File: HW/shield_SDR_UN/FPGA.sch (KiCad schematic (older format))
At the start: 71 parts, among them J1 Conn_02x09_Odd_Even, J2 Conn_02x08_Odd_Even, U4 XC6SLX9-2TQG144C, X2 ASE-xxxMHz

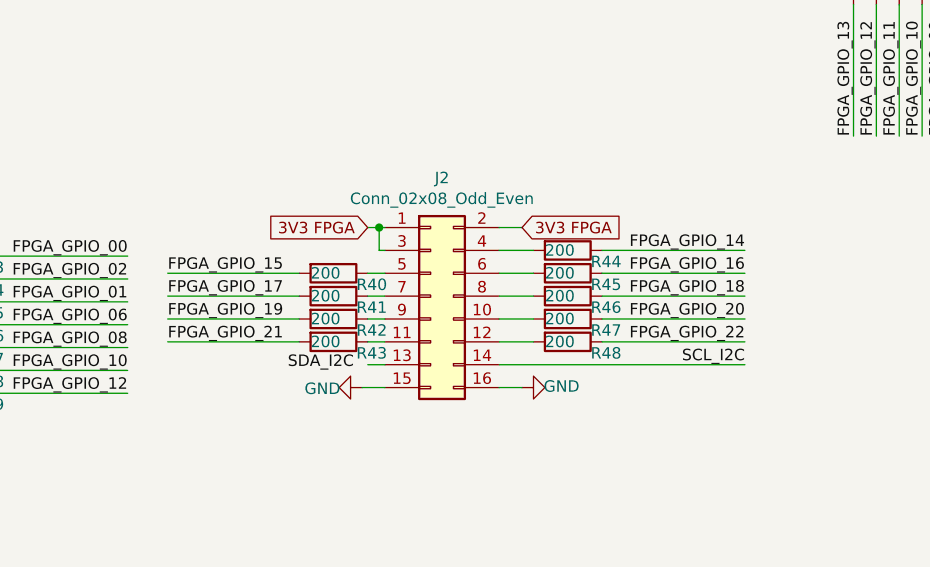
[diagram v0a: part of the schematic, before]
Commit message: organizacion PCB
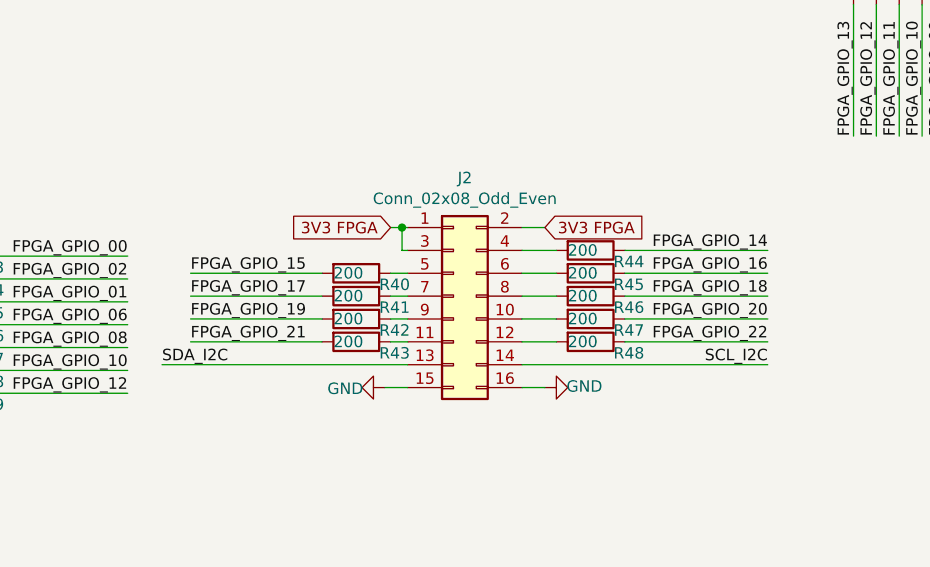
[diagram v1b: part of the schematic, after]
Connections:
- net I2C_SDA: now also J2.13 (Pin_13)
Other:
- moved on the sheet: J2, R40, R41, R42, R43, R44, R45, R46, R47, R48

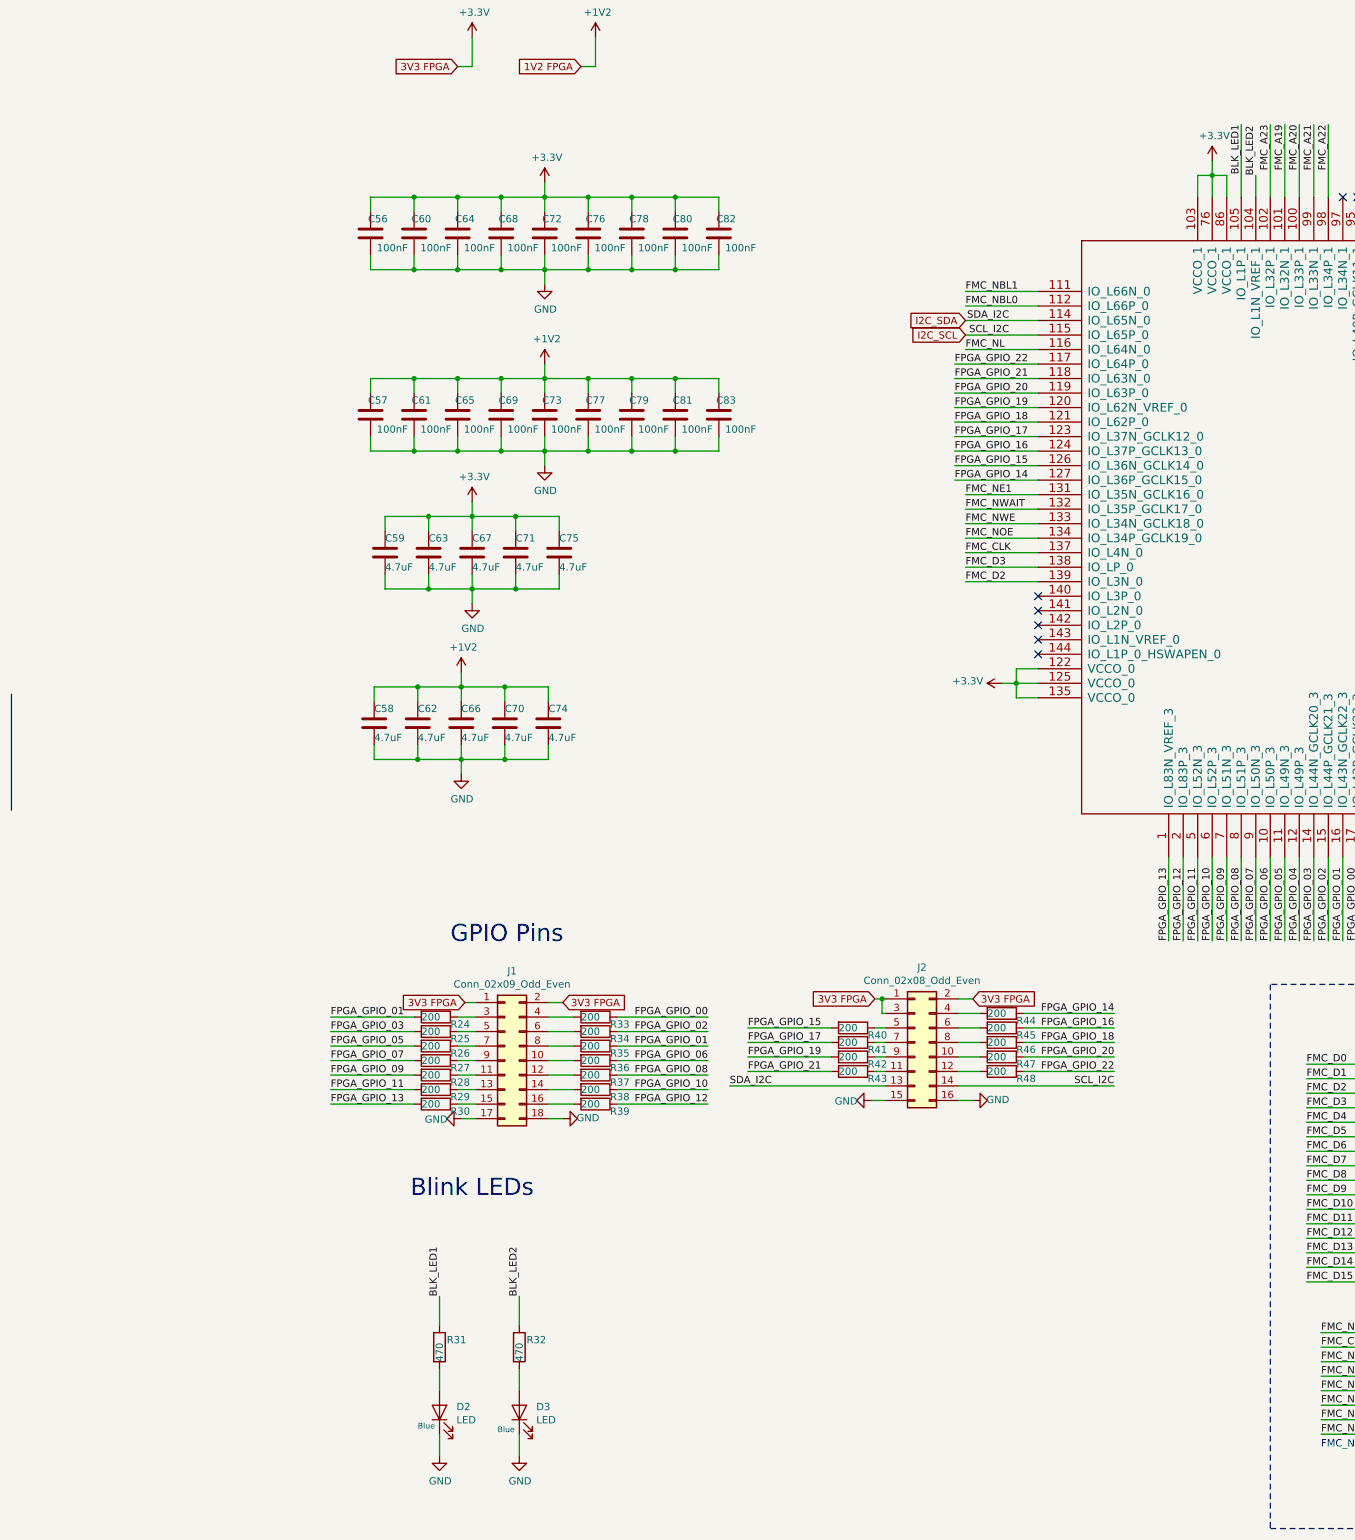
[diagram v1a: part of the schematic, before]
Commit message: organizacion PCB_V2
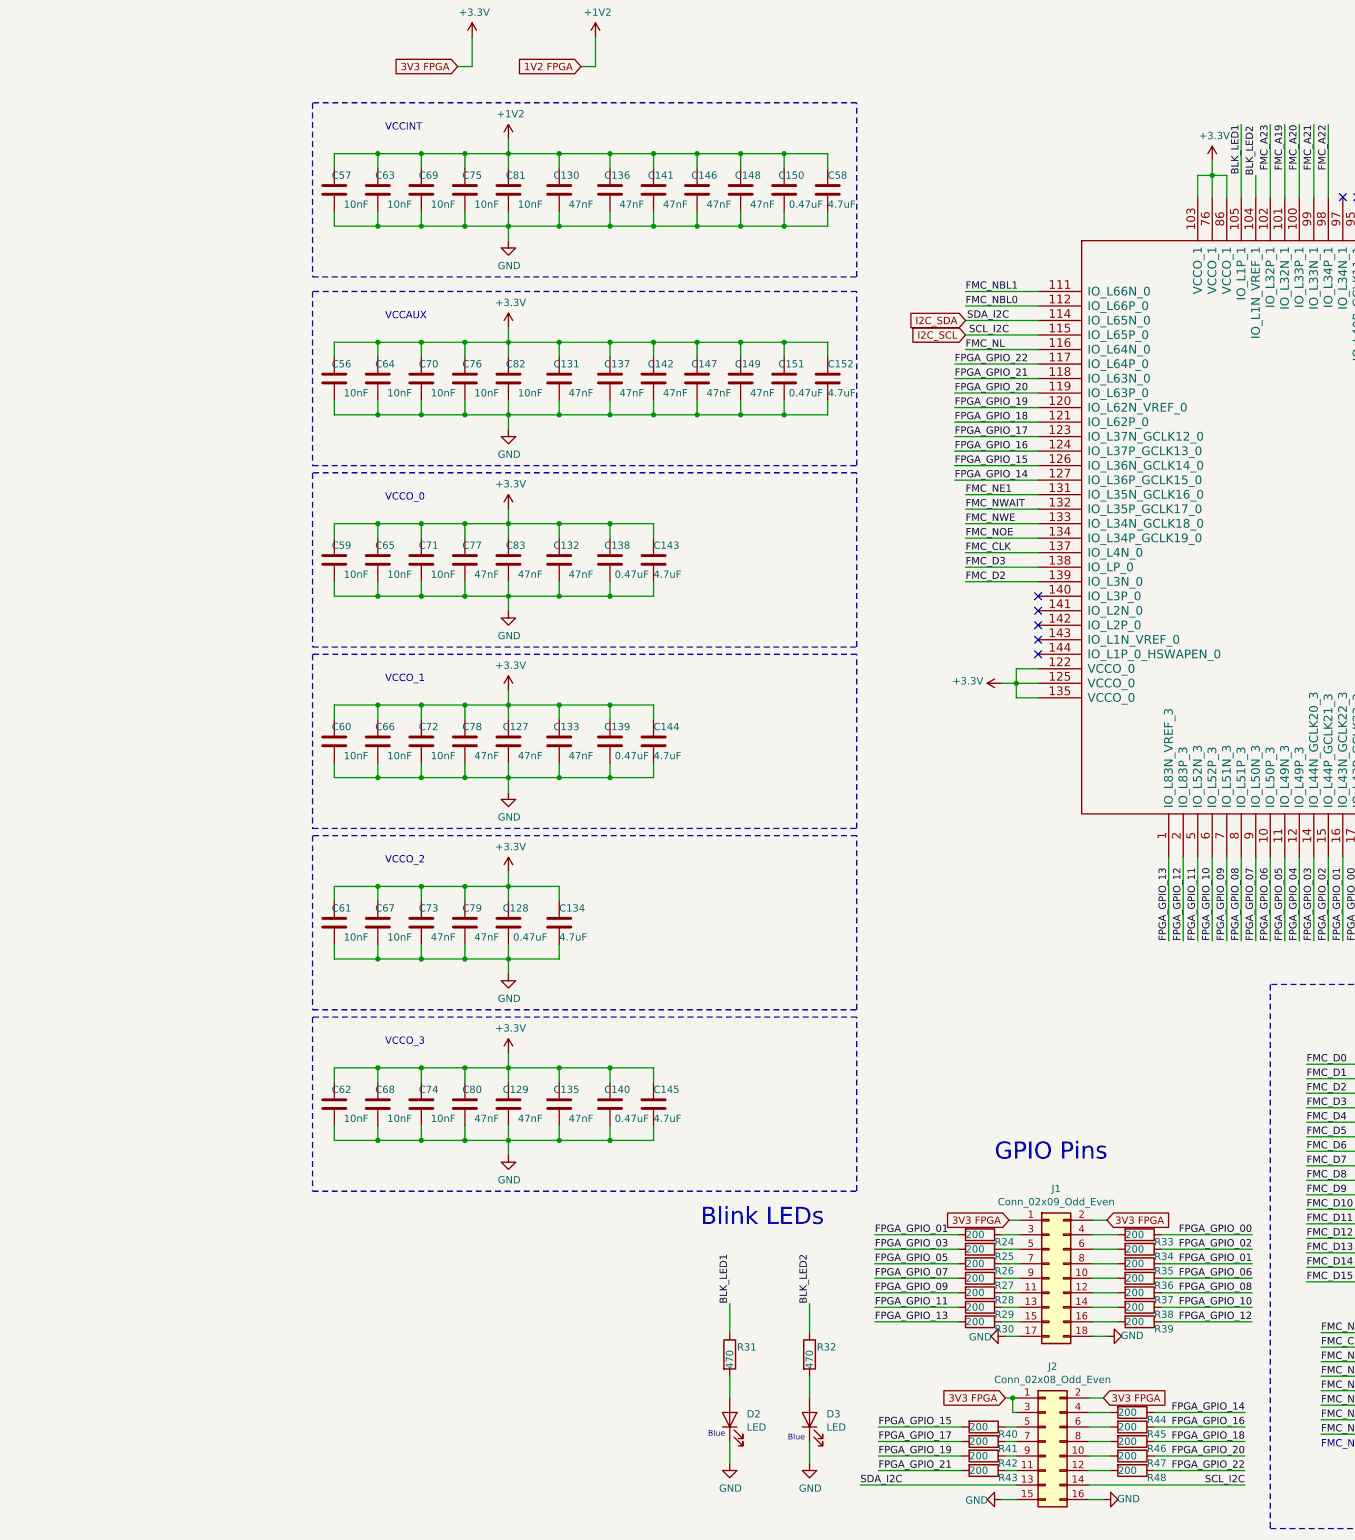
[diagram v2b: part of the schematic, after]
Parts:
- added C127, C129, C130, C131, C132, C133, C135, C136, C137, C141, C142, C146, C147, C148, C149: 47nF, Capacitor_SMD:C_0603_1608Metric_Pad1.05x0.95mm_HandSolder, symbol Device:C
- added C128, C138, C139, C140, C150, C151: 0.47uF, Capacitor_SMD:C_0603_1608Metric_Pad1.05x0.95mm_HandSolder, symbol Device:C
- added C134, C143, C144, C145, C152: 4.7uF, Capacitor_SMD:C_0603_1608Metric_Pad1.05x0.95mm_HandSolder, symbol Device:C
- C56, C57, C60, C61, C64, C65, C68, C69, C72, C76, C81, C82: value 100nF -> 10nF; Digikey 1276-1000-1-ND -> 1276-1009-1-ND
- C59, C62, C63, C66, C67, C70, C71, C74, C75: value 4.7uF -> 10nF; Digikey 1276-1045-1-ND -> 1276-1009-1-ND
- C73, C77, C78, C79, C80, C83: value 100nF -> 47nF; Digikey 1276-1000-1-ND -> 1276-1063-1-ND
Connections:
- net +1V2: now also C63.1, C75.1, C130.1, C136.1, C141.1, C146.1, C148.1, C150.1; no longer C61.1, C62.1, C65.1, C66.1, C70.1, C73.1, C74.1, C77.1, C79.1, C83.1
- net +3V3: now also C61.1, C62.1, C65.1, C66.1, C70.1, C73.1, C74.1, C77.1, C79.1, C83.1, C127.1, C128.1, C129.1, C131.1, C132.1, C133.1, C134.1, C135.1, C137.1, C138.1, C139.1, C140.1, C142.1, C143.1, C144.1, C145.1, C147.1, C149.1, C151.1, C152.1; no longer C63.1, C75.1
- net GND: now also C127.2, C128.2, C129.2, C130.2, C131.2, C132.2, C133.2, C134.2, C135.2, C136.2, C137.2, C138.2, C139.2, C140.2, C141.2, C142.2, C143.2, C144.2, C145.2, C146.2, C147.2, C148.2, C149.2, C150.2, C151.2, C152.2
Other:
- note added: "VCCAUX"
- note added: "VCCINT"
- note added: "VCCO_0"
- note added: "VCCO_1\n"
- note added: "VCCO_2"
- note added: "VCCO_3"
- moved on the sheet: C57, C58, D2, D3, J1, J2, R24, R25, R26, R27, R28, R29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

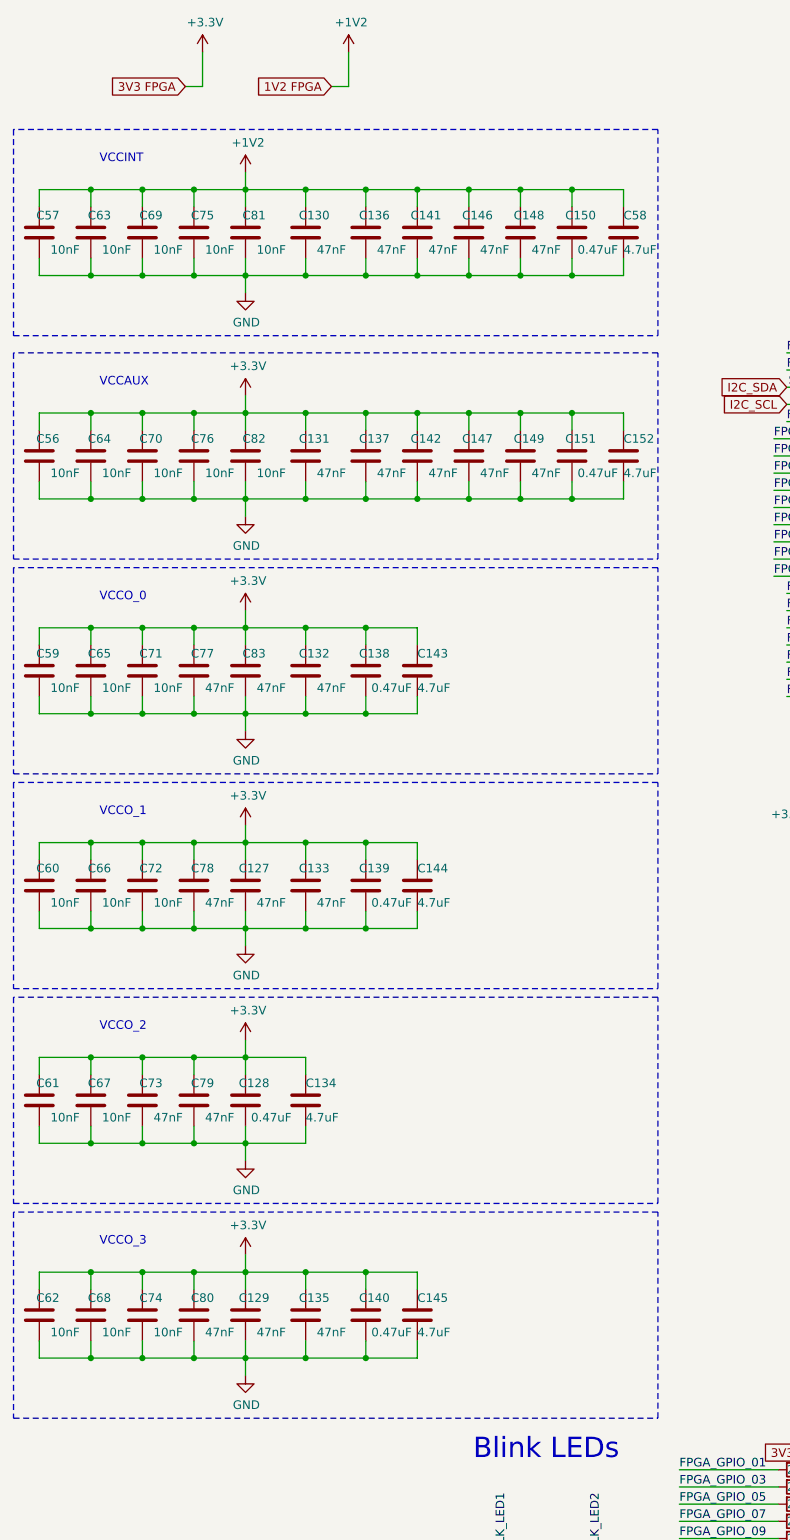
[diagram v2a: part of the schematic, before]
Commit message: organizacion PCB_V3
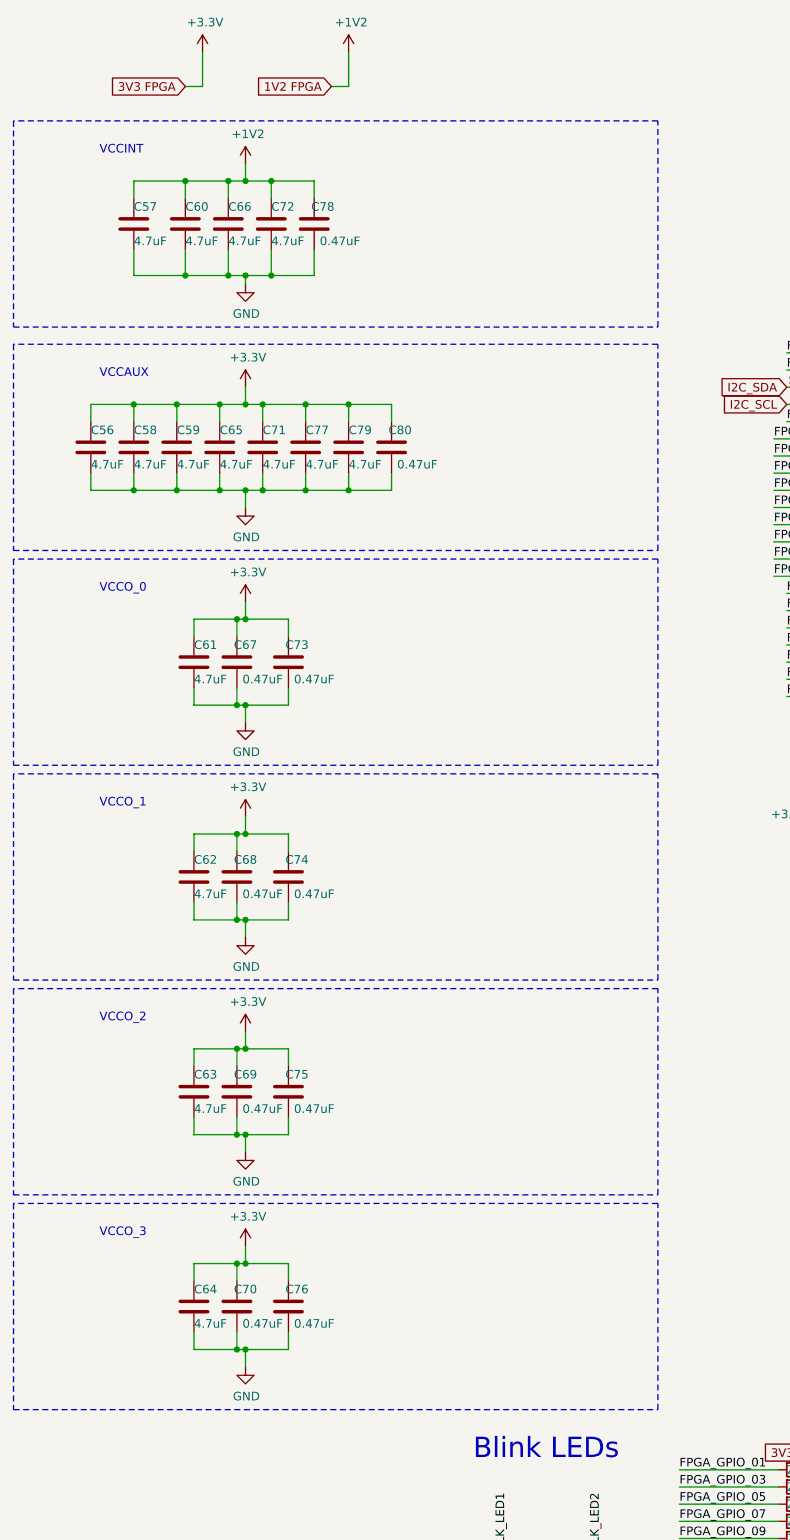
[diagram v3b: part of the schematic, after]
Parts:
- removed C127, C129, C130, C131, C132, C133, C135, C136, C137, C141, C142, C146, C147, C148, C149, C83: 47nF, Capacitor_SMD:C_0603_1608Metric_Pad1.05x0.95mm_HandSolder, symbol Device:C
- removed C128, C138, C139, C140, C150, C151: 0.47uF, Capacitor_SMD:C_0603_1608Metric_Pad1.05x0.95mm_HandSolder, symbol Device:C
- removed C134, C143, C144, C145, C152: 4.7uF, Capacitor_SMD:C_0603_1608Metric_Pad1.05x0.95mm_HandSolder, symbol Device:C
- removed C81, C82: 10nF, Capacitor_SMD:C_0603_1608Metric_Pad1.05x0.95mm_HandSolder, symbol Device:C
- C56, C57, C59, C60, C61, C62, C63, C64, C65, C66, C71, C72: value 10nF -> 4.7uF; Digikey 1276-1009-1-ND -> 1276-1045-1-ND
- C67, C68, C69, C70, C74, C75, C76: value 10nF -> 0.47uF; Digikey 1276-1009-1-ND -> 1276-2082-1-ND
- C73, C78, C80: value 47nF -> 0.47uF; Digikey 1276-1063-1-ND -> 1276-2082-1-ND
- C77, C79: value 47nF -> 4.7uF; Digikey 1276-1063-1-ND -> 1276-1045-1-ND
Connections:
- net +1V2: now also C60.1, C66.1, C72.1, C78.1; no longer C58.1, C63.1, C69.1, C75.1
- net +3V3: now also C58.1, C63.1, C69.1, C75.1; no longer C60.1, C66.1, C72.1, C78.1
